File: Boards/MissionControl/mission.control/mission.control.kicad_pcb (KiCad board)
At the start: 4 copper layers, 41.6 x 31.6 mm, 13 parts, among them U1 E28-2G4M27SX, U2 MAX485_MODULE_5V_LOGIC_TLL_TO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

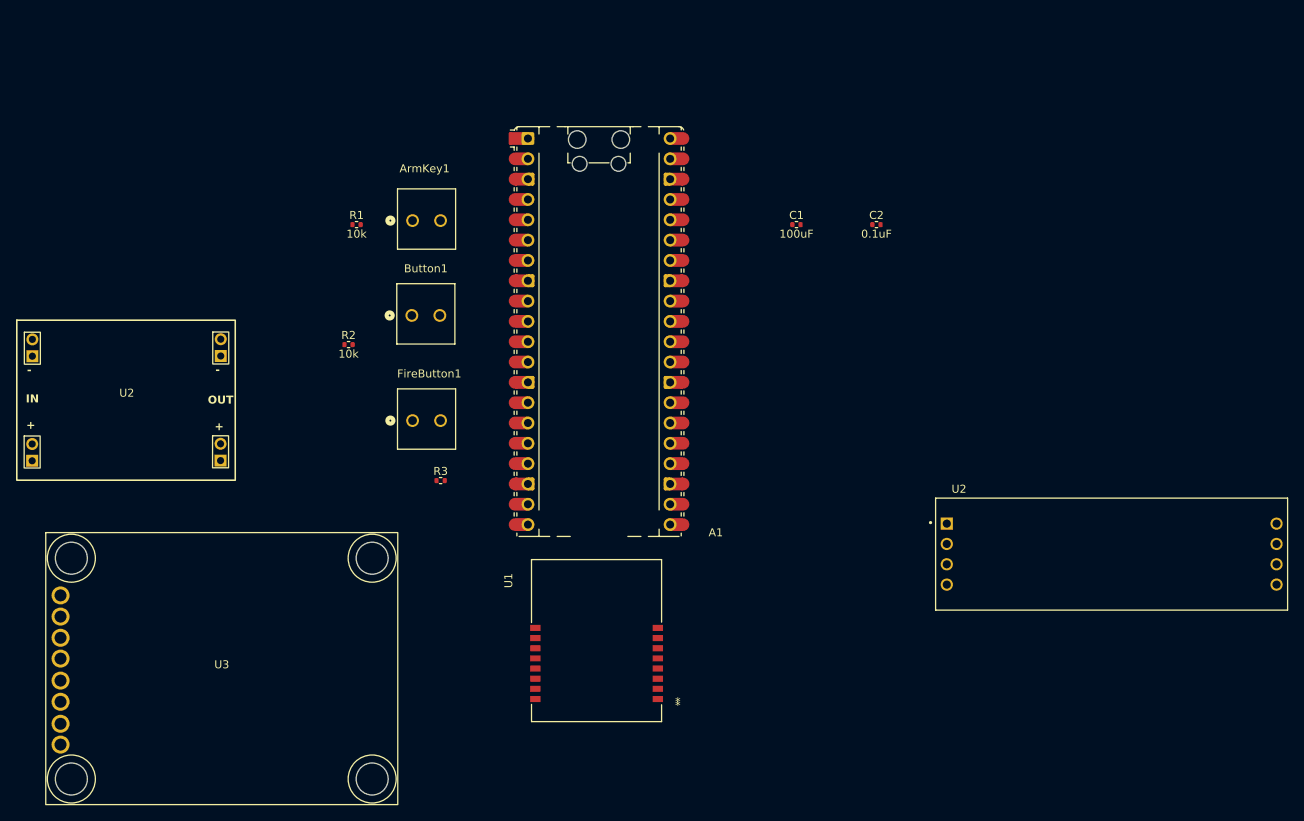
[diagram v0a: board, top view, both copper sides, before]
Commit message: Atualização
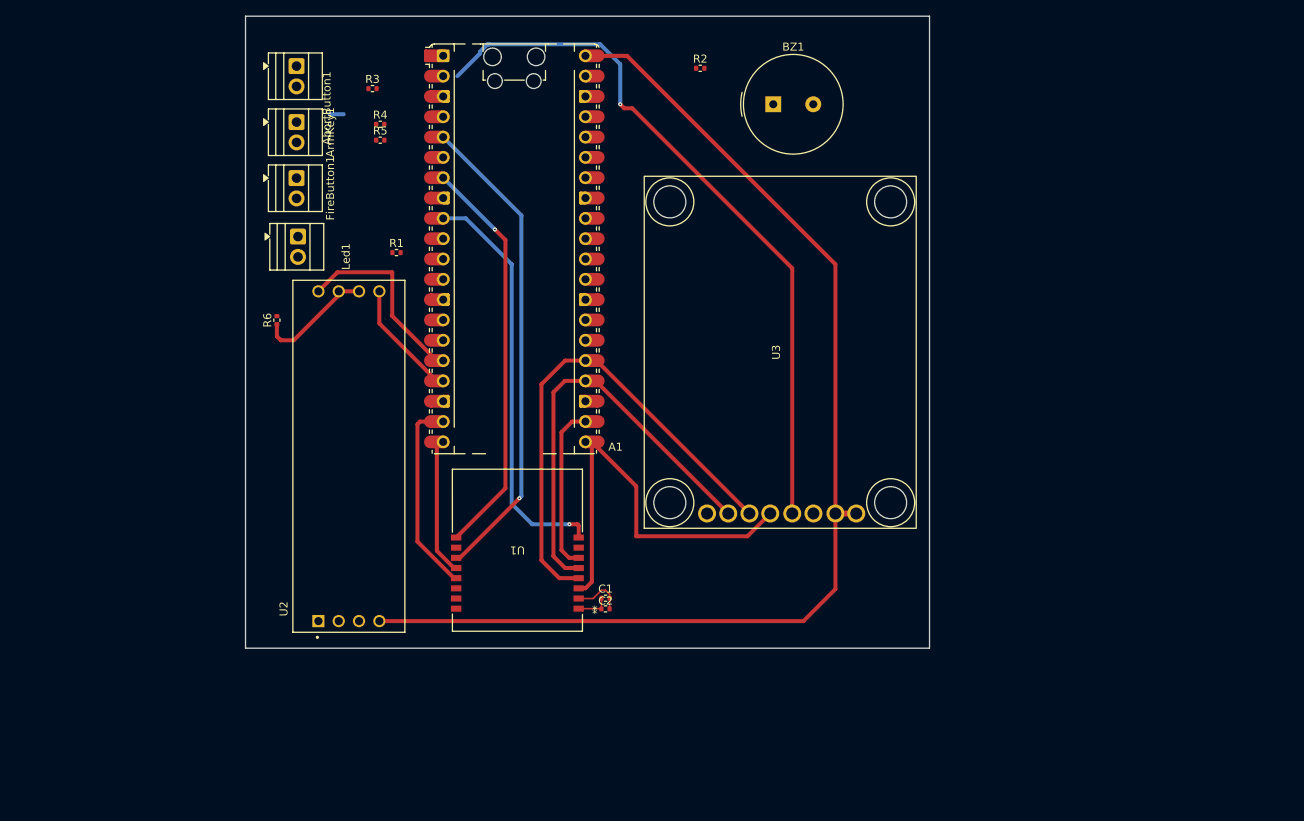
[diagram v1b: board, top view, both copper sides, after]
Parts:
- removed Button1: ., CONN_SD-39357-001_02P_MOL:CONN_SD-39357-001_02P_MOL
- removed the U2 at (88.8, 112.5)
- removed the U2 at (211.9, 132.2)
- added AbortButton1: ., TerminalBlock:TerminalBlock_Xinya_XY308-2.54-2P_1x02_P2.54mm_Horizontal, F.Cu at (110.0, 71.2)
- added BZ1: Buzzer, Buzzer_Beeper:Buzzer_TDK_PS1240P02BT_D12.2mm_H6.5mm, F.Cu at (169.6, 76.0)
- added Led1: ., TerminalBlock:TerminalBlock_Xinya_XY308-2.54-2P_1x02_P2.54mm_Horizontal, F.Cu at (110.2, 92.5)
- added R4: 10KΩ, Resistor_SMD:R_0402_1005Metric, F.Cu at (120.5, 78.5)
- added R5: 10KΩ, Resistor_SMD:R_0402_1005Metric, F.Cu at (120.5, 80.5)
- added R6: 1KΩ, Resistor_SMD:R_0402_1005Metric, F.Cu at (107.5, 103.0)
- added U2: MAX485_MODULE_5V_LOGIC_TLL_TO_RS-485_CONVERTER, MAX485Module:MODULE_MAX485_MODULE_5V_LOGIC_TLL_TO_RS-485_CONVERTER, F.Cu at (116.5, 120.0)
- ArmKey1, FireButton1: footprint CONN_SD-39357-001_02P_MOL:CONN_SD-39357-001_02P_MOL -> TerminalBlock:TerminalBlock_Xinya_XY308-2.54-2P_1x02_P2.54mm_Horizontal
- R1: value 10k -> 220Ω
- R2: value 10k -> 100Ω
- R3: value 10k -> 10KΩ
- moved U3 80.2 mm to (170.5, 107.0), turned to 90 degrees
- moved C2 58.8 mm to (148.6, 139.0)
- moved R2 55.9 mm to (160.5, 71.5)
- moved C1 52.4 mm to (148.6, 137.7)
- moved R3 49.7 mm to (119.5, 74.0)
- moved FireButton1 33.6 mm to (110.0, 85.2), turned to -90 degrees
- moved ArmKey1 19.0 mm to (110.0, 78.2), turned to -90 degrees
- moved U1 15.0 mm to (137.6, 131.7)
- moved A1 14.8 mm to (137.2, 94.0)
- moved R1 6.10 mm to (122.5, 94.5)
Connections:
- A1 pad 1: unconnected-(A1-GPIO0-Pad1) -> /CAN_INT
- A1 pad 10: unconnected-(A1-GPIO7-Pad10) -> /BUZZER_SIGNAL
- A1 pad 11: unconnected-(A1-GPIO8-Pad11) -> /LED_SIGNAL
- A1 pad 12: unconnected-(A1-GPIO9-Pad12) -> /ARM_SIGNAL
- A1 pad 14: unconnected-(A1-GPIO10-Pad14) -> /ABORT_SIGNAL
- A1 pad 15: unconnected-(A1-GPIO11-Pad15) -> /FIRE_SIGNAL
- A1 pad 16: /BUZZER_SIGNAL -> /RS_DI
- A1 pad 17: /RADIO_NRESET -> /RS_RO
- A1 pad 19: /RADIO_BUSY -> /RADIO_DIO1
- A1 pad 2: unconnected-(A1-GPIO1-Pad2) -> /CAN_CS
- A1 pad 20: /RADIO_DIO1 -> /RADIO_BUSY
- A1 pad 21: /RADIO_MISO -> /SPI0_MISO
- A1 pad 24: /RADIO_SCK -> /SPI0_SCK
- A1 pad 25: /RADIO_MOSI -> /SPI0_MOSI
- A1 pad 29: unconnected-(A1-GPIO22-Pad29) -> /RS_DE
- A1 pad 4: unconnected-(A1-GPIO2-Pad4) -> /BUZZER_SIGNAL
- A1 pad 5: unconnected-(A1-GPIO3-Pad5) -> /RADIO_NRESET
- A1 pad 7: unconnected-(A1-GPIO5-Pad7) -> /RADIO_TX_EN
- A1 pad 9: unconnected-(A1-GPIO6-Pad9) -> /RADIO_RX_EN
- R1 pad 2: GND -> /LED_SIGNAL
- R2 pad 1: Net-(Button1-Pin_2) -> /BUZZER_SIGNAL
- R2 pad 2: GND -> Net-(BZ1-+)
- R3 pad 1: Net-(Button2-Pin_2) -> GND
- R3 pad 2: GND -> /FIRE_SIGNAL
- U1 pad 3: /RADIO_MISO -> /SPI0_MISO
- U1 pad 4: /RADIO_MOSI -> /SPI0_MOSI
- U1 pad 5: /RADIO_SCK -> /SPI0_SCK
- U3 pad 2: /CAN_SCK -> /SPI0_SCK
- U3 pad 3: unconnected-(U3-SI-Pad3) -> /SPI0_MOSI
- U3 pad 4: unconnected-(U3-SO-Pad4) -> /SPI0_MISO
- U3 pad 5: unconnected-(U3-CS-Pad5) -> /CAN_CS
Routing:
- net +5V: track 0.00 -> 143.1 mm
- net /CAN_CS: track 0.00 -> 90.6 mm, vias 0 -> 1
- net /SPI0_MOSI: track 0.00 -> 61.9 mm
- net /RADIO_NRESET: track 0.00 -> 60.3 mm, vias 0 -> 1
- net /SPI0_SCK: track 0.00 -> 52.8 mm
- net /SPI0_MISO: track 0.00 -> 52.6 mm
- net /RADIO_RX_EN: track 0.00 -> 52.0 mm, vias 0 -> 1
- net /RADIO_TX_EN: track 0.00 -> 50.8 mm, vias 0 -> 1
- net /RADIO_DIO1: track 0.00 -> 24.0 mm
- net /RS_DI: track 0.00 -> 23.6 mm
- net /RADIO_CS: track 0.31 -> 20.9 mm
- net /RADIO_BUSY: track 0.00 -> 16.9 mm
- net /RS_TXEN: track 0.00 -> 14.3 mm
- net /RS_RO: track 0.00 -> 14.2 mm
- net GND: track 0.00 -> 6.81 mm
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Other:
- board size 41.6 x 31.6 mm -> 85.5 x 79 mm

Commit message: Atualização
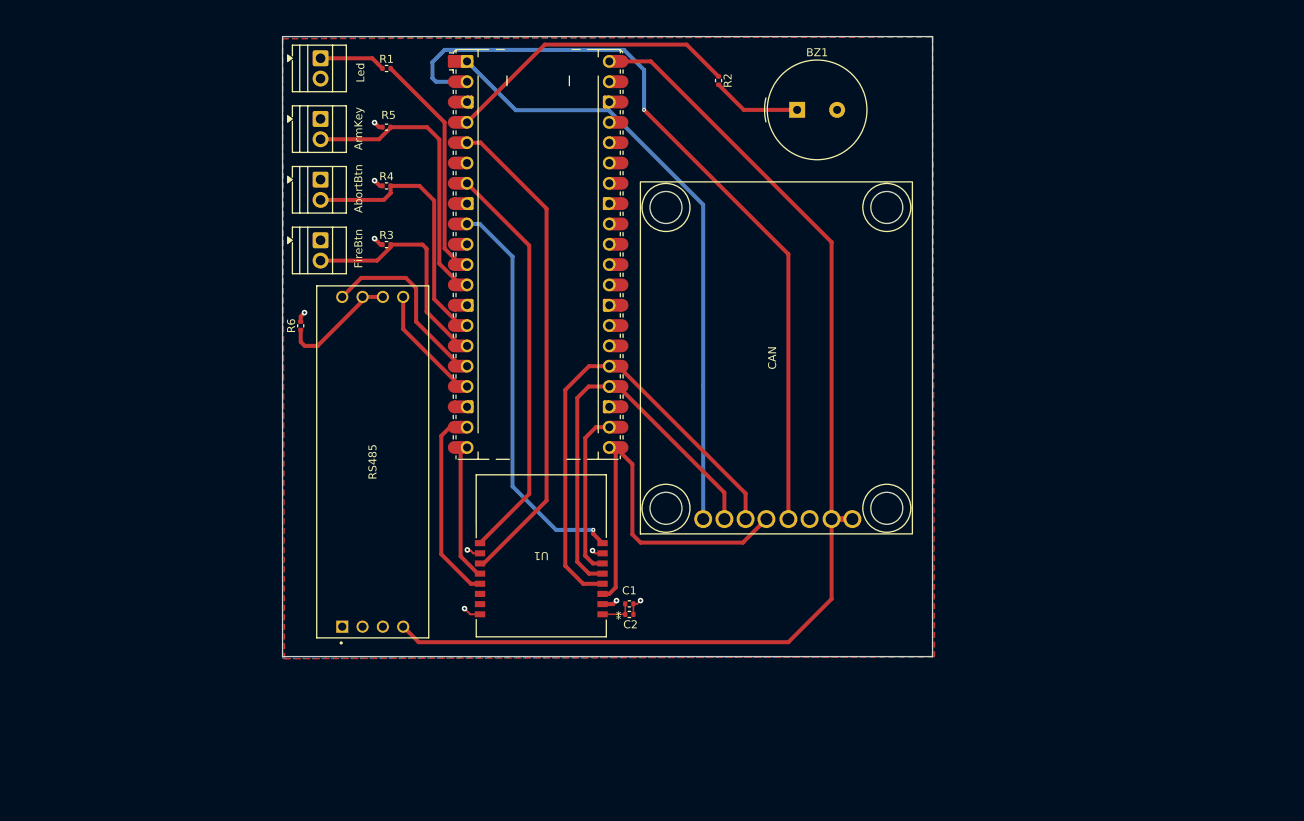
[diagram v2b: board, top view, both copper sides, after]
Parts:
- moved R1 23.0 mm to (121.2, 71.5)
- moved Led 22.5 mm to (113.0, 70.2)
- moved R3 19.6 mm to (121.2, 93.5)
- moved AbortBtn 14.5 mm to (113.0, 85.4)
- moved FireBtn 8.33 mm to (113.0, 93.0)
- moved R4 7.74 mm to (121.2, 86.2)
- moved BZ1 3.06 mm to (172.6, 76.7)
- moved C2 3.06 mm to (151.6, 139.7)
- moved A1 3.06 mm to (140.2, 94.7)
- moved R6 3.06 mm to (110.5, 103.7)
- moved RS485 3.06 mm to (119.5, 120.7)
- moved C1 3.06 mm to (151.6, 138.4)
- moved U1 3.06 mm to (140.6, 132.4)
- moved ArmKey 3.03 mm to (113.0, 77.8)
- moved R2 2.76 mm to (162.8, 73.0), turned to -90 degrees
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- renumbered AbortButton1 to AbortBtn, ArmKey1 to ArmKey, U3 to CAN, FireButton1 to FireBtn, Led1 to Led, U2 to RS485
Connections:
- A1 pad 36: unconnected-(A1-3V3-Pad36) -> +3.3V
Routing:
- net /CAN_INT: track 0.00 -> 76.2 mm
- net /BUZZER_SIGNAL: track 0.00 -> 37.1 mm
- net /ARM_SIGNAL: track 0.00 -> 35.4 mm
- net /ABORT_SIGNAL: track 0.00 -> 33.2 mm
- net /FIRE_SIGNAL: track 0.00 -> 29.2 mm
- net /LED_SIGNAL: track 0.00 -> 28.1 mm
- net Net-(BZ1-+): track 0.00 -> 11.1 mm
- net Net-(Led1-Pin_1): track 0.00 -> 8.27 mm
- net GND: track 6.81 -> 14.8 mm, vias 0 -> 9
- net /CAN_CS: track 90.6 -> 98.3 mm
- net +5V: track 143.1 -> 140.1 mm
- net /SPI0_MISO: track 52.6 -> 50.7 mm
- net /RADIO_RX_EN: track 52.0 -> 50.6 mm
- net /RADIO_NRESET: track 60.3 -> 61.4 mm, vias 1 -> 0
- net /RS_DI: track 23.6 -> 22.8 mm
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- added copper zone on F.Cu, net +3.3V
- added copper zone on B.Cu, net GND
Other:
- board size 85.5 x 79 mm -> 81.2 x 77.5 mm
- copper layers 4 -> 2
